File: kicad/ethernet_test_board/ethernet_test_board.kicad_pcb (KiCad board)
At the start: 2 copper layers, 100 x 100 mm, 0 parts

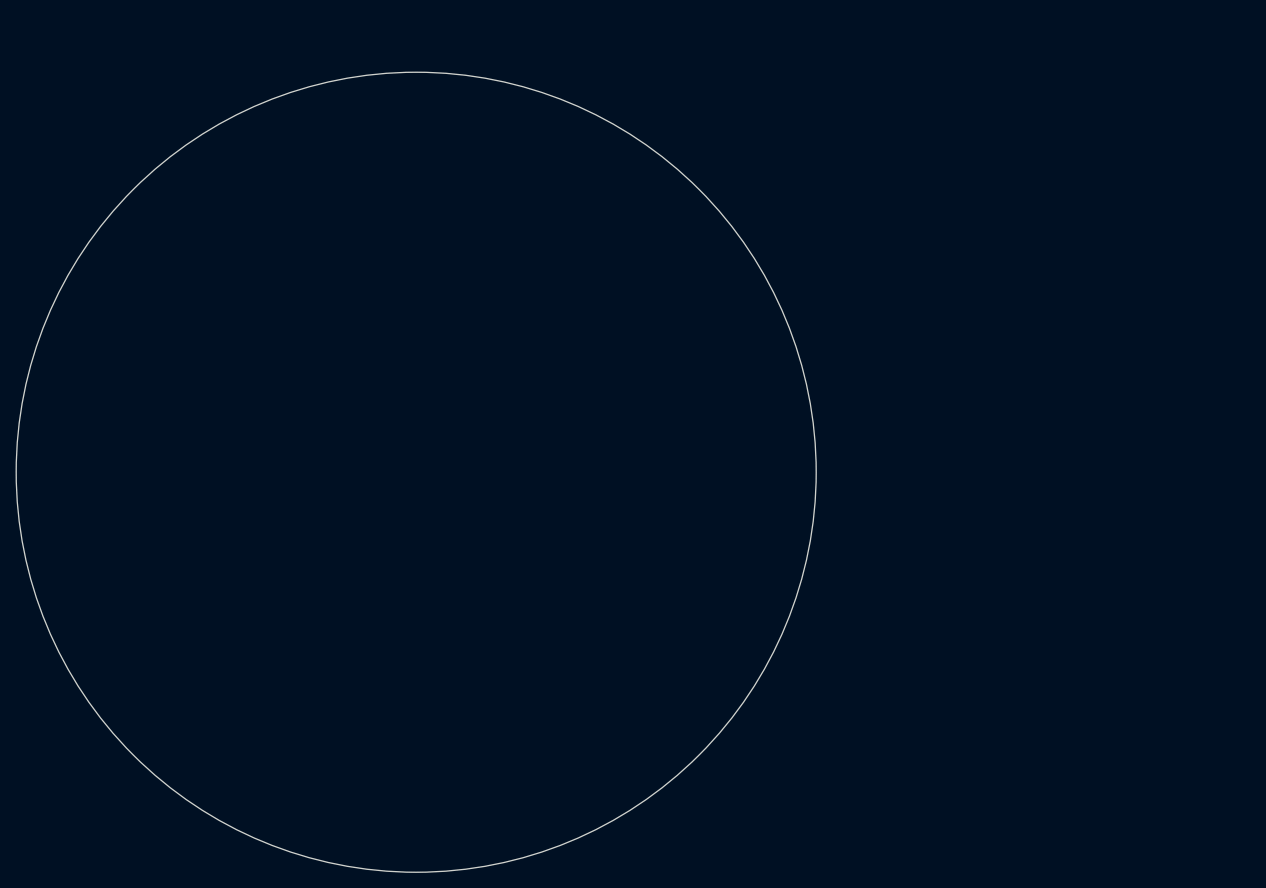
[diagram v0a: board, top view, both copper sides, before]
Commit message: [add] kicad sch (finish) kicad pcb (WIP)
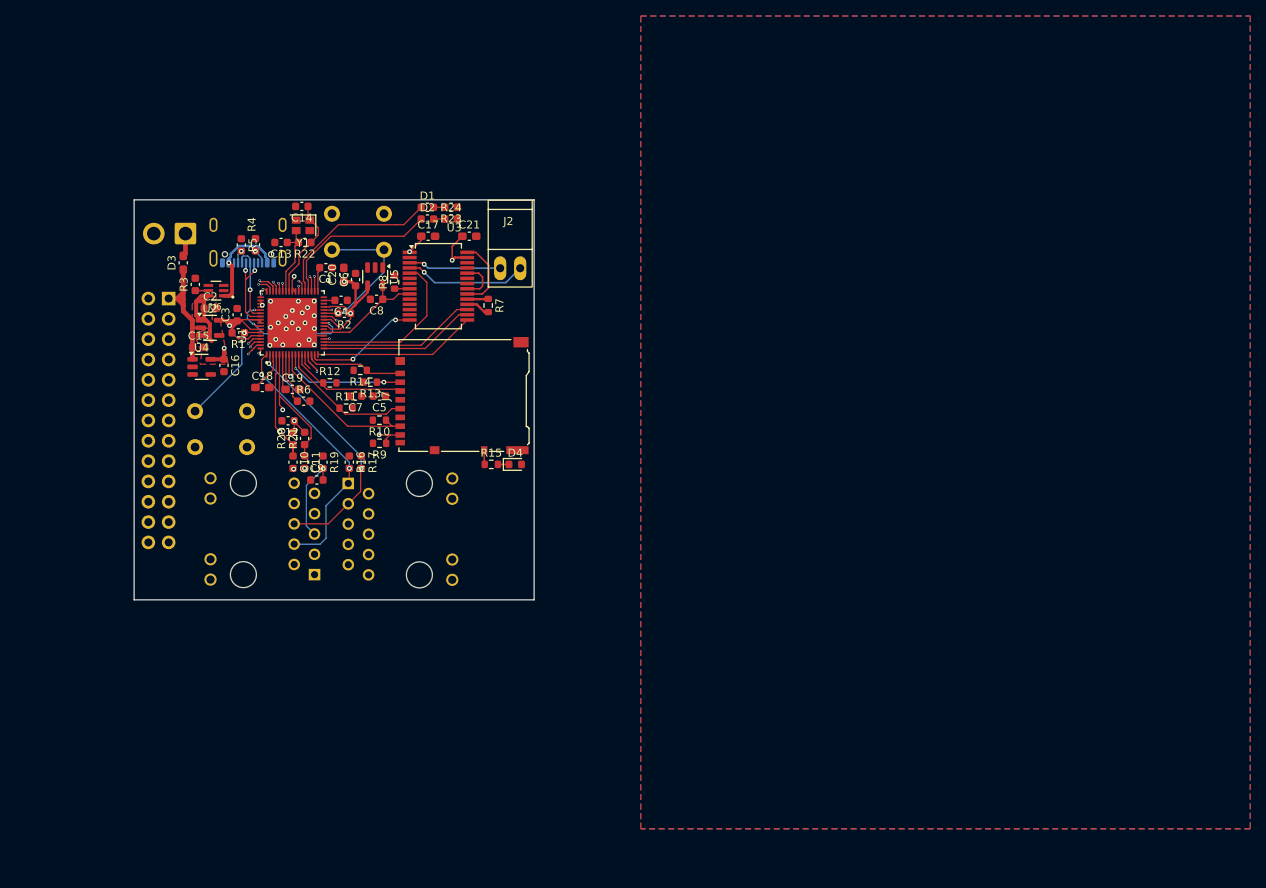
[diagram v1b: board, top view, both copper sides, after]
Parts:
- added C1: 10nF, Capacitor_SMD:C_0603_1608Metric, F.Cu at (138.7, 54.4)
- added C10: 6.8n, Capacitor_SMD:C_0603_1608Metric, F.Cu at (134.6, 78.7)
- added C11: 6.8n, Capacitor_SMD:C_0603_1608Metric, F.Cu at (136.1, 78.7)
- added C12: 10n, Capacitor_SMD:C_0603_1608Metric, F.Cu at (134.0, 73.6)
- added C13: 18p, Capacitor_SMD:C_0603_1608Metric, F.Cu at (133.1, 51.3)
- added C14: 18p, Capacitor_SMD:C_0603_1608Metric, F.Cu at (135.7, 46.8)
- added C15: 1μ, Capacitor_SMD:C_0603_1608Metric, F.Cu at (122.8, 64.4)
- added C16: 1μ, Capacitor_SMD:C_0603_1608Metric, F.Cu at (126.0, 66.7)
- added C17: C, Capacitor_SMD:C_0603_1608Metric_Pad1.08x0.95mm_HandSolder, F.Cu at (151.5, 50.5)
- added C18: C, Capacitor_SMD:C_0603_1608Metric_Pad1.08x0.95mm_HandSolder, F.Cu at (130.8, 69.4)
- added C19: C, Capacitor_SMD:C_0603_1608Metric_Pad1.08x0.95mm_HandSolder, F.Cu at (134.5, 69.6)
- added C2: 10μ, Capacitor_SMD:C_0603_1608Metric, F.Cu at (124.3, 59.5)
- added C20: C, Capacitor_SMD:C_0603_1608Metric_Pad1.08x0.95mm_HandSolder, F.Cu at (140.9, 55.3)
- added C21: C, Capacitor_SMD:C_0603_1608Metric_Pad1.08x0.95mm_HandSolder, F.Cu at (156.6, 50.5)
- added C3: 10μ, Capacitor_SMD:C_0603_1608Metric, F.Cu at (127.6, 60.3)
- added C4: 4.7μ, Capacitor_SMD:C_0603_1608Metric, F.Cu at (140.6, 58.5)
- added C5: 0.1μ, Capacitor_SMD:C_0603_1608Metric, F.Cu at (145.4, 70.5)
- added C6: 0.1u, Capacitor_SMD:C_0603_1608Metric, F.Cu at (142.4, 55.9)
- added C7: 10μ, Capacitor_SMD:C_0603_1608Metric, F.Cu at (142.4, 70.5)
- added C8: 15p, Capacitor_SMD:C_0603_1608Metric, F.Cu at (145.0, 58.4)
- added C9: 22n, Capacitor_SMD:C_0603_1608Metric, F.Cu at (137.6, 81.0)
- added D1: LED, Capacitor_SMD:C_0603_1608Metric, F.Cu at (151.4, 46.9)
- added D2: LED, Capacitor_SMD:C_0603_1608Metric, F.Cu at (151.4, 48.4)
- added D3: D, Capacitor_SMD:C_0603_1608Metric_Pad1.08x0.95mm_HandSolder, F.Cu at (120.9, 53.8)
- added D4: LED, LED_SMD:LED_0603_1608Metric, F.Cu at (162.4, 79.0)
- added J1: USB_C_Receptacle_USB2.0_16P, Connector_USB:USB_C_Receptacle_GCT_USB4105-xx-A_16P_TopMnt_Horizontal, B.Cu at (129.0, 50.2)
- added J2: Conn_01x02_Pin, ILG:ILG2pin, F.Cu at (161.8, 54.5)
- added J3: TMJD4152NENLC, TMJD4152NENLC:TMJD4152NENLC, B.Cu at (141.5, 81.4)
- added J4: Conn_02x13_Top_Bottom, Connector_PinHeader_2.54mm:PinHeader_2x13_P2.54mm_Vertical, B.Cu at (119.1, 58.3)
- added J5: TMJD4152NENLC, TMJD4152NENLC:TMJD4152NENLC, B.Cu at (137.3, 92.8)
- added J7: Micro_SD_Card_Det_Hirose_DM3AT, Connector_Card:microSD_HC_Hirose_DM3AT-SF-PEJM5, F.Cu at (155.7, 70.4)
- added J8: Conn_01x02_Pin, Connector_JST:JST_VH_B2P-VH-B_1x02_P3.96mm_Vertical, B.Cu at (121.2, 50.2)
- added R1: 1k, Capacitor_SMD:C_0603_1608Metric, F.Cu at (127.8, 62.6)
- added R10: 10K, Resistor_SMD:R_0603_1608Metric, F.Cu at (145.4, 73.5)
- added R11: 10K, Resistor_SMD:R_0603_1608Metric, F.Cu at (141.2, 72.0)
- added R12: 10K, Resistor_SMD:R_0603_1608Metric, F.Cu at (139.2, 68.8)
- added R13: 10K, Resistor_SMD:R_0603_1608Metric, F.Cu at (144.3, 68.7)
- added R14: 10K, Resistor_SMD:R_0603_1608Metric, F.Cu at (143.0, 67.3)
- added R15: 100, Resistor_SMD:R_0603_1608Metric, F.Cu at (159.4, 79.0)
- added R16: 49.9, Capacitor_SMD:C_0603_1608Metric, F.Cu at (141.6, 78.7)
- added R17: 49.9, Capacitor_SMD:C_0603_1608Metric, F.Cu at (143.1, 78.8)
- added R19: 10, Capacitor_SMD:C_0603_1608Metric, F.Cu at (138.3, 78.8)
- added R2: R, Capacitor_SMD:C_0603_1608Metric, F.Cu at (141.0, 60.1)
- added R20: 49.9, Capacitor_SMD:C_0603_1608Metric, F.Cu at (134.6, 75.8)
- added R21: 49.9, Capacitor_SMD:C_0603_1608Metric, F.Cu at (136.1, 75.8)
- added R22: 1M, Capacitor_SMD:C_0603_1608Metric, F.Cu at (136.1, 51.3)
- added R23: R, Capacitor_SMD:C_0603_1608Metric, F.Cu at (154.4, 46.9)
- added R24: R, Capacitor_SMD:C_0603_1608Metric, F.Cu at (154.4, 48.4)
- added R3: R, Capacitor_SMD:C_0603_1608Metric, F.Cu at (122.4, 56.5)
- added R4: 5.1k, Capacitor_SMD:C_0603_1608Metric, F.Cu at (129.9, 51.6)
- added R5: 5.1k, Capacitor_SMD:C_0603_1608Metric, F.Cu at (128.1, 51.6)
- added R6: 12.4k, Capacitor_SMD:C_0603_1608Metric, F.Cu at (135.9, 71.1)
- added R7: 10k, Resistor_SMD:R_0603_1608Metric, F.Cu at (159.0, 59.2)
- added R8: 1k, Resistor_SMD:R_0603_1608Metric, F.Cu at (147.3, 56.2)
- added R9: 10K, Resistor_SMD:R_0603_1608Metric, F.Cu at (145.4, 76.4)
- added SW1: SW_Push, Button_Switch_THT:SW_PUSH_6mm_H7.3mm, B.Cu at (146.0, 47.7)
- added SW2: SW_Push, Button_Switch_THT:SW_PUSH_6mm_H7.3mm, B.Cu at (122.4, 76.9)
- added U1: W55RP20, W55RP20:QFN40P800X800X90-69N, F.Cu at (134.5, 61.3)
- added U2: RT9080, Package_TO_SOT_SMD:TSOT-23-5, F.Cu at (124.2, 62.0)
- added U3: MCP25625-x-SS, Package_SO:SSOP-28_5.3x10.2mm_P0.65mm, F.Cu at (152.8, 56.7)
- added U4: XC6201, Package_TO_SOT_SMD:SOT-23-5, F.Cu at (123.2, 66.8)
- added U5: SiT2001B, Package_TO_SOT_SMD:SOT-23-5, F.Cu at (144.9, 55.6)
- added U6: LM66100DCKR, LM66100DCKR:SOT65P210X110-6N, F.Cu at (125.0, 57.3)
- added Y1: FA-128, Oscillator:Oscillator_SMD_SeikoEpson_SG210-4Pin_2.5x2.0mm, F.Cu at (135.8, 49.1)
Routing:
- net +3.3V: track 0.00 -> 105.0 mm, vias 0 -> 7
- net /SPEED: track 0.00 -> 67.8 mm, vias 0 -> 1
- net +5V: track 0.00 -> 67.3 mm, vias 0 -> 2
- net /TXM: track 0.00 -> 55.6 mm, vias 0 -> 2
- net /TXP: track 0.00 -> 55.0 mm, vias 0 -> 2
- net GND: track 0.00 -> 51.8 mm, vias 0 -> 22
- net /Ethernet_PoE: track 0.00 -> 44.4 mm
- net /SWD: track 0.00 -> 42.6 mm, vias 0 -> 1
- net /SWCLK: track 0.00 -> 39.1 mm, vias 0 -> 1
- net /RXP: track 0.00 -> 39.0 mm, vias 0 -> 1
- net Net-(J3-CT_2): track 0.00 -> 38.4 mm, vias 0 -> 1
- net /RXM: track 0.00 -> 36.4 mm, vias 0 -> 1
- net /GPIO16: track 0.00 -> 33.7 mm, vias 0 -> 1
- net /GPIO15: track 0.00 -> 30.6 mm, vias 0 -> 1
- net /GPIO18: track 0.00 -> 26.1 mm, vias 0 -> 1
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- added copper zone on F.Cu, net +5V
- added copper zone on B.Cu, net GND
- added copper zone on F.Cu, net GND
- added copper zone on In1.Cu, net GND
- added copper zone on In2.Cu, net GND
- added copper zone on In3.Cu, net GND
- added copper zone on In4.Cu, net GND
- added copper zone on In5.Cu, net GND
- added copper zone on In6.Cu, net GND
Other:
- board size 100 x 100 mm -> 50 x 50 mm
- copper layers 2 -> 8
